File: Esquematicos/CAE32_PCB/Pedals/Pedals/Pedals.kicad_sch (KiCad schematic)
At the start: 19 parts, among them J1 SPI_MASTER, J2 CAN, J3 PGRM and SPI, SW1 CONFIG, SW2 BOOT, SW3 RST, U1 STM32F072RBTx

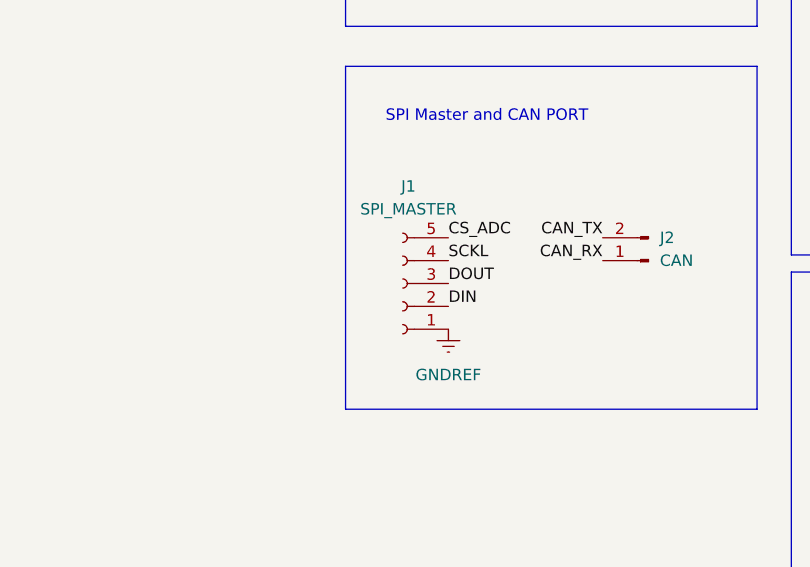
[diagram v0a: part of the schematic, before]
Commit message: chore: arrange schematics components
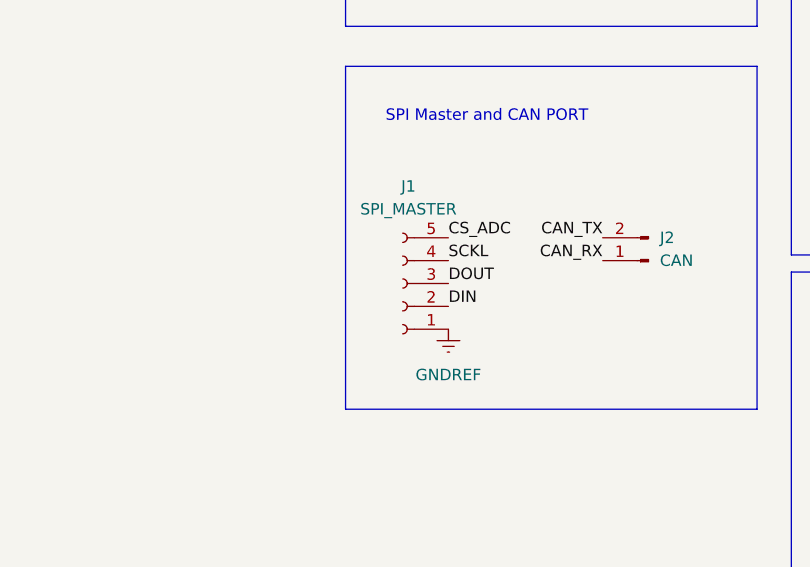
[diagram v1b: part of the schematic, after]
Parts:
- C1: footprint Capacitor_SMD:C_0603_1608Metric_Pad1.08x0.95mm_HandSolder -> Capacitor_SMD:C_0603_1608Metric
- D1, D2, D3: footprint LED_SMD:LED_0805_2012Metric_Pad1.15x1.40mm_HandSolder -> LED_SMD:LED_0805_2012Metric
- R1, R2, R3, R4: footprint Resistor_SMD:R_0603_1608Metric_Pad0.98x0.95mm_HandSolder -> Resistor_SMD:R_0603_1608Metric
